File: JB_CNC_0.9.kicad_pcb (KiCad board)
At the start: 2 copper layers, 80 parts, among them CON1 POWER_IN, J1 Arduino_Nano_Header, P1 Z_CTRL, P10 X_LIMIT_1, P11 Y_LIMIT_1, P12 Z_LIMIT_1, P13 FLUIDO, P14 X_LIMIT_2, P15 Y_LIMIT_2, P16 Z_LIMIT_2, P17 SPINDLE_PWR, P18 SPINDLE_LED_ON, P19 SPINDLE_DIRECTION, P2 Z_LIMIT, P20 RESET/ABORT, P21 START/RESUME, P22 FEED_HOLD, P23 SAFETY_DOOR, P24 ASPIRADOR, P25 earth, P26 SPINDLE_LED_OFF, P3 Y_CTRL, P4 Y_LIMIT, P5 X_CTRL, P6 X_LIMIT, P7 USB_TO_ARDUINO, P8 F_INV, P9 USB_SHIELD_INPUT, Q1 BC546, Q2 BC546, Q3 BC546, Q4 BC546, Q5 BC546, U1 CA3140, U2 LM7805CT, U3 CA3140, U4 74LS86

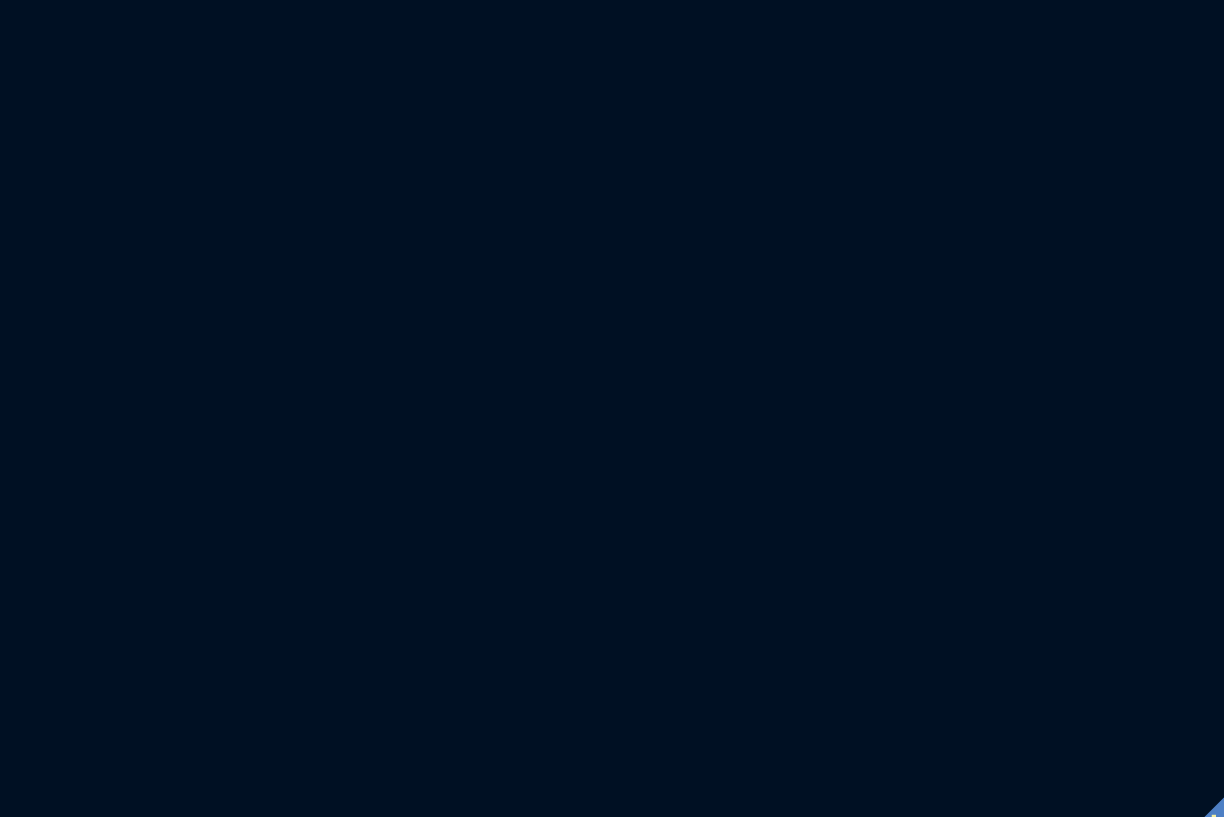
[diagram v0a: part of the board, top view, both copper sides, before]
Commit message: Desenho da placa em andamento
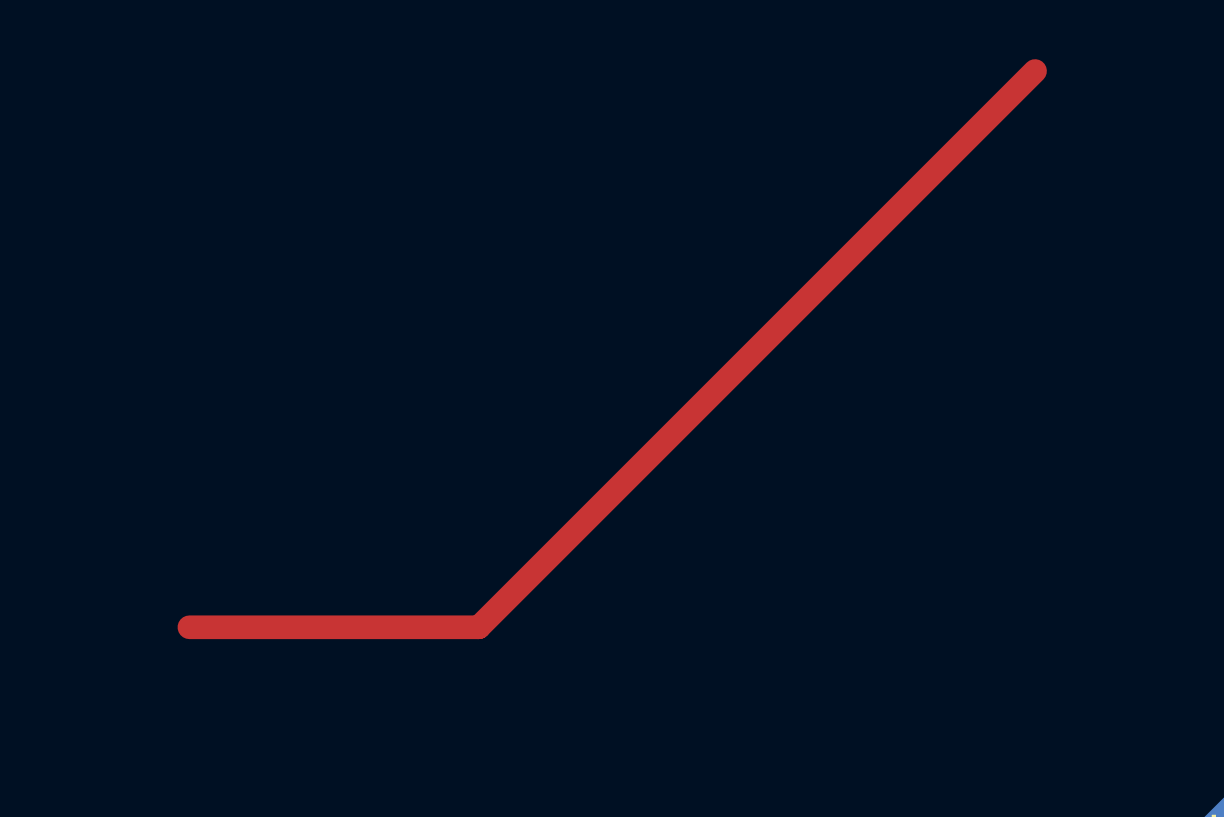
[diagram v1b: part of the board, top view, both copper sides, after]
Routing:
- net (no net): track 0.00 -> 36.4 mm
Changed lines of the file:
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@@
     (links 172)
     (no_connects 81)
-    (area -128.705 -22.48 240.765001 182.9212)
+    (area -128.705 22.98346 274.083451 149.54)
     (thickness 1.6)
     (drawings 4)
-    (tracks 638)
+    (tracks 640)
     (zones 0)
     (modules 80)
@@
   (gr_line (start 240.665 132.715) (end 240.665 42.545) (angle 90) (layer F.Fab) (width 0.2))
   (gr_line (start 50.8 132.715) (end 240.665 132.715) (angle 90) (layer F.Fab) (width 0.2))
+  (segment (start 20.701 42.799) (end 30.48 42.799) (width 0.8) (layer F.Cu) (net 0))
+  (segment (start 30.48 42.799) (end 49.276 24.003) (width 0.8) (layer F.Cu) (net 0))
   (segment (start 159.258 67.945) (end 161.29 67.945) (width 1.4) (layer B.Cu) (net 2))
   (segment (start 166.497 62.738) (end 169.037 62.738) (width 1.4) (layer B.Cu) (net 2))

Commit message: primeiro commit colaborativo
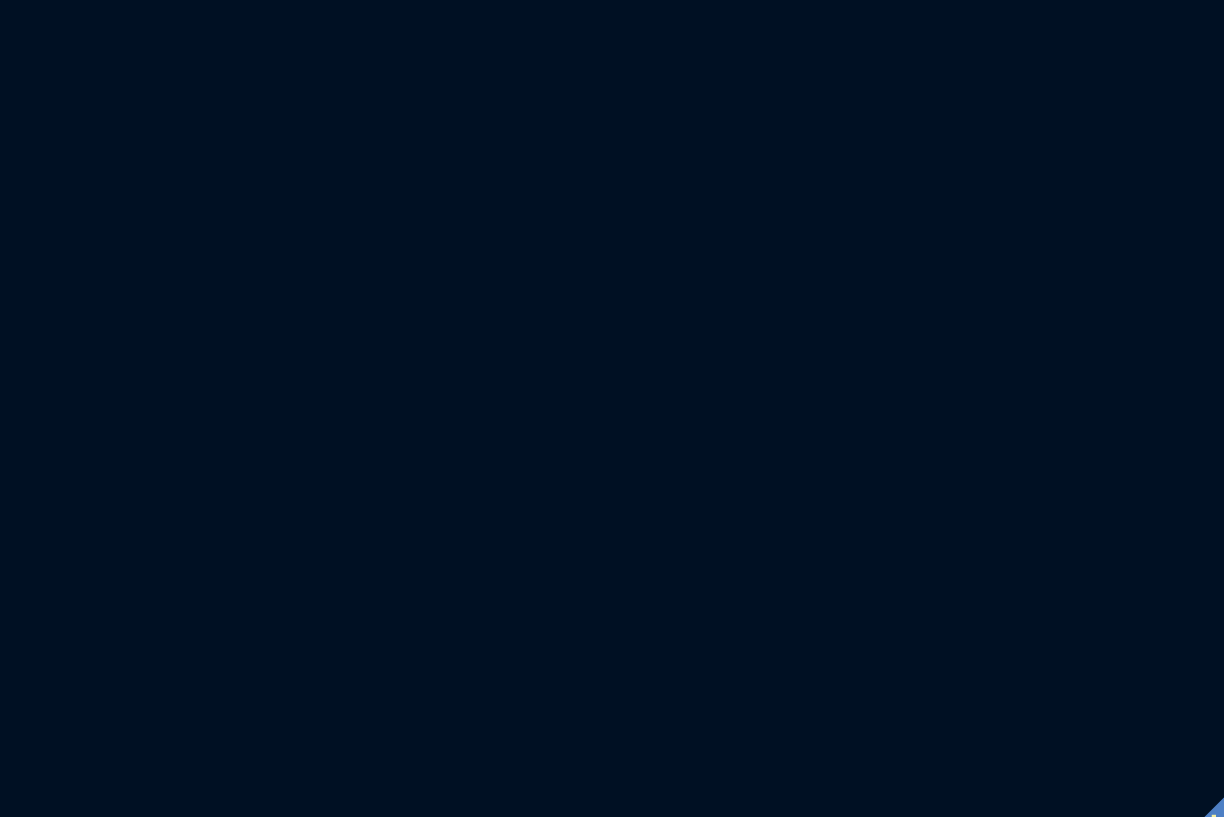
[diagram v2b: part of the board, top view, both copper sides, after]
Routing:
- net (no net): track 36.4 -> 0.00 mm
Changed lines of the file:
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@@
-(kicad_pcb (version 4) (host pcbnew 4.0.2+dfsg1-2~bpo8+1-stable)
+(kicad_pcb (version 4) (host pcbnew 4.0.2-stable)
   (general
     (links 172)
@@
     (thickness 1.6)
     (drawings 4)
-    (tracks 640)
+    (tracks 638)
     (zones 0)
     (modules 80)
@@
   (gr_line (start 240.665 132.715) (end 240.665 42.545) (angle 90) (layer F.Fab) (width 0.2))
   (gr_line (start 50.8 132.715) (end 240.665 132.715) (angle 90) (layer F.Fab) (width 0.2))
-  (segment (start 20.701 42.799) (end 30.48 42.799) (width 0.8) (layer F.Cu) (net 0))
-  (segment (start 30.48 42.799) (end 49.276 24.003) (width 0.8) (layer F.Cu) (net 0))
   (segment (start 159.258 67.945) (end 161.29 67.945) (width 1.4) (layer B.Cu) (net 2))
   (segment (start 166.497 62.738) (end 169.037 62.738) (width 1.4) (layer B.Cu) (net 2))
